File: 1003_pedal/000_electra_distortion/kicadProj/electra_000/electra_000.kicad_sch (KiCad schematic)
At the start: 17 parts, among them J1 AudioJack2, J2 AudioJack2, Q1 Q_NPN_BCE, SW1 SW_Slide_DPDT

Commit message: schematic
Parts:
- C1, C2, C3: KiLib_Generator (none) -> capacitor/THT/other
- D1, D2, D3, D4: KiLib_Generator (none) -> diode/THT
- R1, R3: KiLib_Generator (none) -> resistor/THT
- R2: footprint Resistor_THT:R_Axial_DIN0207_L6.3mm_D2.5mm_P7.62mm_Horizontal -> Resistor_THT:R_Axial_DIN0207_L6.3mm_D2.5mm_P2.54mm_Vertical; KiLib_Generator (none) -> resistor/THT
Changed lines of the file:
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@@
+			)
+		)
+		(property "KiLib_Generator" "capacitor/THT/other"
+			(at 163.83 44.45 0)
+			(hide yes)
+			(show_name no)
+			(do_not_autoplace no)
+			(effects
+				(font
+					(size 1.27 1.27)
+				)
 			)
 		)
@@
 			)
 		)
+		(property "KiLib_Generator" "resistor/THT"
+			(at 129.54 110.49 0)
+			(hide yes)
+			(show_name no)
+			(do_not_autoplace no)
+			(effects
+				(font
+					(size 1.27 1.27)
+				)
+			)
+		)
 		(pin "2"
 		)
@@
 			)
 		)
+		(property "KiLib_Generator" "diode/THT"
+			(at 152.4 83.82 0)
+			(hide yes)
+			(show_name no)
+			(do_not_autoplace no)
+			(effects
+				(font
+					(size 1.27 1.27)
+				)
+			)
+		)
 		(pin "1"
 		)
@@
 			)
 		)
+		(property "KiLib_Generator" "resistor/THT"
+			(at 129.54 58.42 0)
+			(hide yes)
+			(show_name no)
+			(do_not_autoplace no)
+			(effects
+				(font
+					(size 1.27 1.27)
+				)
+			)
+		)
 		(pin "1"
 		)
@@
 			)
 		)
+		(property "KiLib_Generator" "capacitor/THT/other"
+			(at 163.83 66.04 0)
+			(hide yes)
+			(show_name no)
+			(do_not_autoplace no)
+			(effects
+				(font
+					(size 1.27 1.27)
+				)
+			)
+		)
 		(pin "1"
 		)
@@
 			)
 		)
+		(property "KiLib_Generator" "diode/THT"
+			(at 152.4 97.79 0)
+			(hide yes)
+			(show_name no)
+			(do_not_autoplace no)
+			(effects
+				(font
+					(size 1.27 1.27)
+				)
+			)
+		)
 		(pin "1"
 		)
@@
 			)
 		)
+		(property "KiLib_Generator" "capacitor/THT/other"
+			(at 143.51 62.23 0)
+			(hide yes)
+			(show_name no)
+			(do_not_autoplace no)
+			(effects
+				(font
+					(size 1.27 1.27)
+				)
+			)
+		)
 		(pin "1"
 		)
@@
 			)
 		)
-		(property "Footprint" "Resistor_THT:R_Axial_DIN0207_L6.3mm_D2.5mm_P7.62mm_Horizontal"
+		(property "Footprint" "Resistor_THT:R_Axial_DIN0207_L6.3mm_D2.5mm_P2.54mm_Vertical"
 			(at 125.73 64.008 90)
 			(hide yes)
@@
 			)
 		)
+		(property "KiLib_Generator" "resistor/THT"
+			(at 125.73 62.23 0)
+			(hide yes)
+			(show_name no)
+			(do_not_autoplace no)
+			(effects
+				(font
+					(size 1.27 1.27)
+				)
+			)
+		)
 		(pin "2"
 		)
@@
 			)
 		)
+		(property "KiLib_Generator" "diode/THT"
+			(at 152.4 78.74 0)
+			(hide yes)
+			(show_name no)
+			(do_not_autoplace no)
+			(effects
+				(font
+					(size 1.27 1.27)
+				)
+			)
+		)
 		(pin "1"
 		)
@@
 			(at 152.4 106.68 0)
 			(hide yes)
+			(show_name no)
+			(do_not_autoplace no)
+			(effects
+				(font
+					(size 1.27 1.27)
+				)
+			)
+		)
+		(property "KiLib_Generator" "diode/THT"
+			(at 152.4 106.68 0)
+			(hide yes)

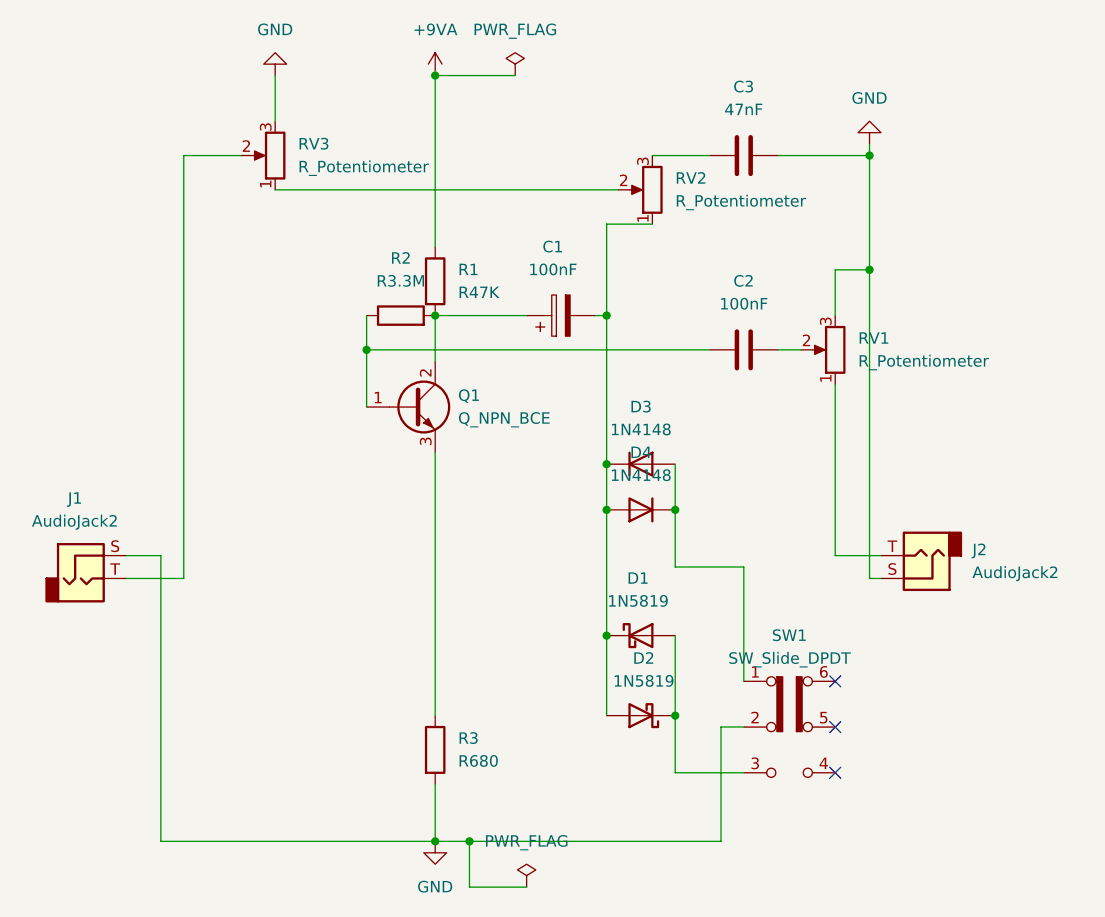
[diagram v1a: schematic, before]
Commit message: layout
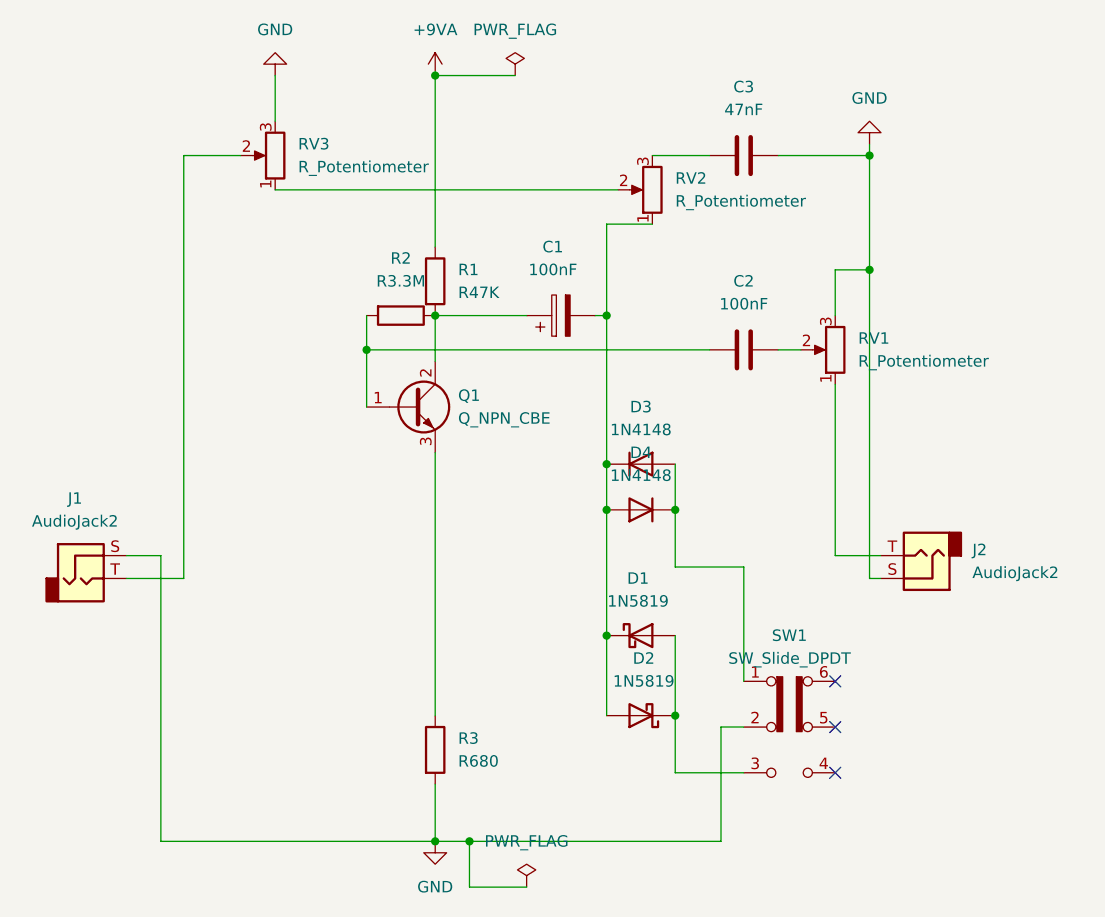
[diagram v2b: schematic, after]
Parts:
- D1, D2: footprint Diode_THT:D_DO-41_SOD81_P10.16mm_Horizontal -> Diode_THT:D_DO-41_SOD81_P7.62mm_Horizontal
- Q1: value Q_NPN_BCE -> Q_NPN_CBE; footprint Package_TO_SOT_THT:TO-92_Inline -> Monkey_Riot_Pedals_Library:TO-92L_INLINE_WIDE
- R1: footprint Resistor_THT:R_Axial_DIN0207_L6.3mm_D2.5mm_P7.62mm_Horizontal -> Resistor_THT:R_Axial_DIN0204_L3.6mm_D1.6mm_P7.62mm_Horizontal
- R2: footprint Resistor_THT:R_Axial_DIN0207_L6.3mm_D2.5mm_P2.54mm_Vertical -> Resistor_THT:R_Axial_DIN0204_L3.6mm_D1.6mm_P2.54mm_Vertical
- R3: footprint Resistor_THT:R_Axial_DIN0207_L6.3mm_D2.5mm_P7.62mm_Horizontal -> Resistor_THT:R_Axial_DIN0309_L9.0mm_D3.2mm_P12.70mm_Horizontal
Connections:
- net at C2.1, Q1.1 (B): now also R2.2; no longer R2.1
- net at C1.1, Q1.2 (C), R1.2: now also R2.1; no longer R2.2
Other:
- moved on the sheet: R2
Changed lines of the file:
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@@
+	(wire
+		(pts
+			(xy 121.92 66.04) (xy 160.02 66.04)
+		)
+		(stroke
+			(width 0)
+			(type default)
+		)
+	)
 	(wire
 		(pts
@@
 		(pts
 			(xy 148.59 62.23) (xy 148.59 78.74)
-		)
-		(stroke
-			(width 0)
-			(type default)
-		)
-	)
-	(wire
-		(pts
-			(xy 160.02 66.04) (xy 121.92 66.04)
 		)
 		(stroke
@@
 			)
 		)
-		(property "Footprint" "Resistor_THT:R_Axial_DIN0207_L6.3mm_D2.5mm_P7.62mm_Horizontal"
+		(property "Footprint" "Resistor_THT:R_Axial_DIN0309_L9.0mm_D3.2mm_P12.70mm_Horizontal"
 			(at 127.762 110.49 90)
 			(hide yes)
@@
 			)
 		)
-		(property "Value" "Q_NPN_BCE"
+		(property "Value" "Q_NPN_CBE"
 			(at 132.08 73.6599 0)
 			(show_name no)
@@
 			)
 		)
-		(property "Footprint" "Package_TO_SOT_THT:TO-92_Inline"
+		(property "Footprint" "Monkey_Riot_Pedals_Library:TO-92L_INLINE_WIDE"
 			(at 132.08 69.85 0)
 			(hide yes)
@@
 			)
 		)
-		(property "Footprint" "Resistor_THT:R_Axial_DIN0207_L6.3mm_D2.5mm_P7.62mm_Horizontal"
+		(property "Footprint" "Resistor_THT:R_Axial_DIN0204_L3.6mm_D1.6mm_P7.62mm_Horizontal"
 			(at 127.762 58.42 90)
 			(hide yes)
@@
 			)
 		)
-		(property "Footprint" "Diode_THT:D_DO-41_SOD81_P10.16mm_Horizontal"
+		(property "Footprint" "Diode_THT:D_DO-41_SOD81_P7.62mm_Horizontal"
 			(at 152.4 102.235 0)
 			(hide yes)
@@
 	(symbol
 		(lib_id "Device:R")
-		(at 125.73 62.23 90)
+		(at 125.73 62.23 270)
 		(unit 1)
 		(body_style 1)
@@
 			)
 		)
-		(property "Footprint" "Resistor_THT:R_Axial_DIN0207_L6.3mm_D2.5mm_P2.54mm_Vertical"
-			(at 125.73 64.008 90)
+		(property "Footprint" "Resistor_THT:R_Axial_DIN0204_L3.6mm_D1.6mm_P2.54mm_Vertical"
+			(at 125.73 60.452 90)
 			(hide yes)
 			(show_name no)
@@
 			)
 		)
-		(property "Footprint" "Diode_THT:D_DO-41_SOD81_P10.16mm_Horizontal"
+		(property "Footprint" "Diode_THT:D_DO-41_SOD81_P7.62mm_Horizontal"
 			(at 152.4 102.235 0)
 			(hide yes)

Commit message: pcb update
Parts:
- R3: footprint Resistor_THT:R_Axial_DIN0309_L9.0mm_D3.2mm_P12.70mm_Horizontal -> Resistor_THT:R_Axial_DIN0207_L6.3mm_D2.5mm_P10.16mm_Horizontal
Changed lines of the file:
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@@
 			)
 		)
-		(property "Footprint" "Resistor_THT:R_Axial_DIN0309_L9.0mm_D3.2mm_P12.70mm_Horizontal"
+		(property "Footprint" "Resistor_THT:R_Axial_DIN0207_L6.3mm_D2.5mm_P10.16mm_Horizontal"
 			(at 127.762 110.49 90)
 			(hide yes)
